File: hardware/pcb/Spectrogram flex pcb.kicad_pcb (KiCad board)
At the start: 2 copper layers, 153.2 x 54.5 mm, 10 parts

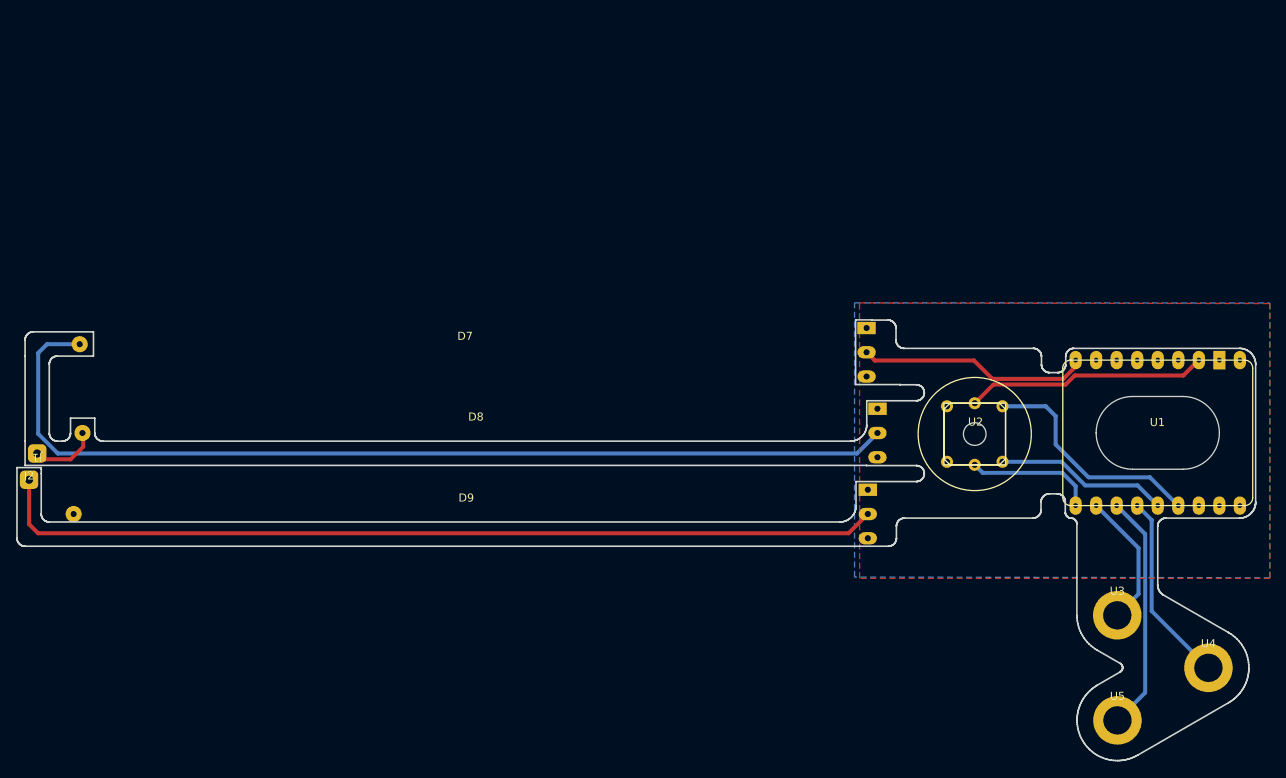
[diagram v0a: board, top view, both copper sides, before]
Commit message: PCB revision
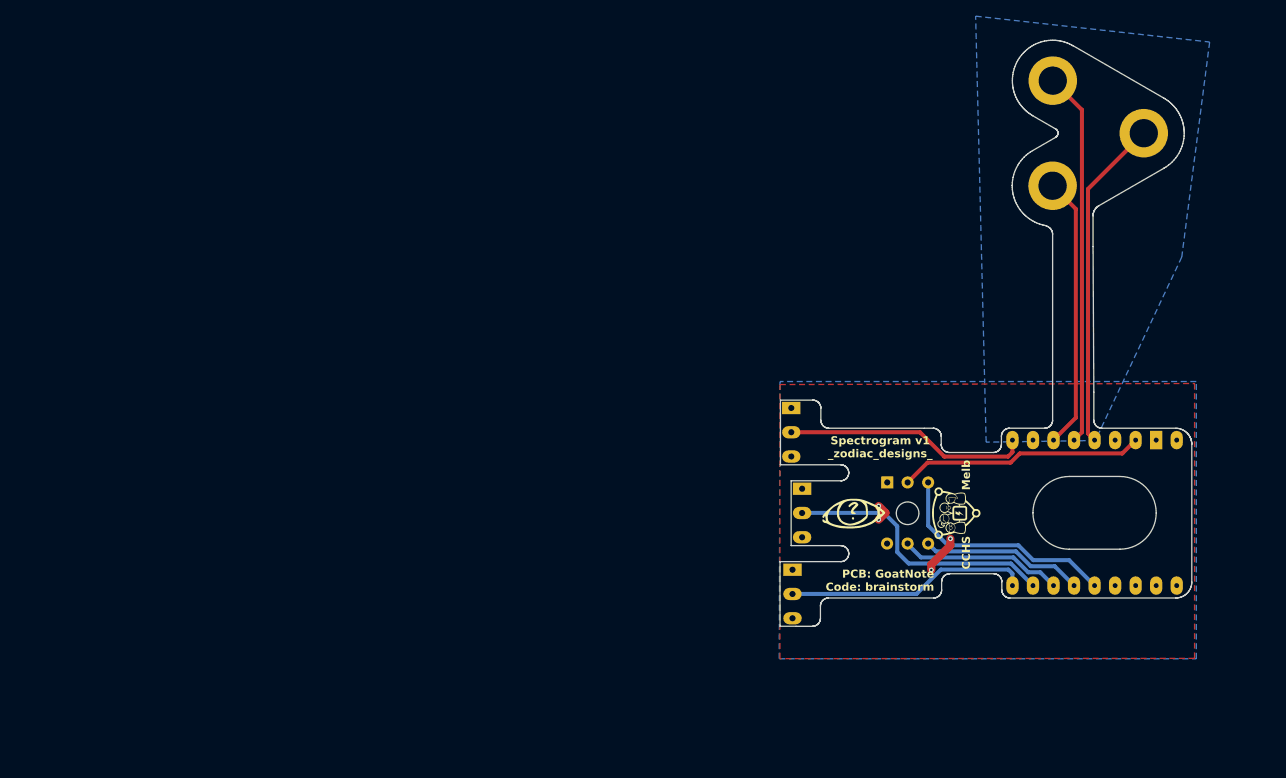
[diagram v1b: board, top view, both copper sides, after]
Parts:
- removed J1, J2: ~, Waveshare_ESP32_S3_mini:jumper pad
- added G***: LOGO, LOGO, F.Cu at (194.7, 79.2)
- added G***: LOGO, LOGO, F.Cu at (181.9, 79.4)
- added G***: LOGO, LOGO, B.Cu at (211.1, 32.4)
- moved U5 79.5 mm to (206.6, 25.7)
- moved U4 66.6 mm to (217.9, 32.2)
- moved U3 53.7 mm to (206.6, 38.7)
- moved D7 13.6 mm to (74.9, 65.2)
- moved D9 13.6 mm to (75.1, 85.2)
- moved D8 13.6 mm to (76.3, 75.2)
- moved U2 12.8 mm to (188.7, 79.2)
- moved U1 12.6 mm to (223.6, 70.1)
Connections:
- net +5V renamed Net-(D7-5V)
- D8 pad 3: Net-(D7-Dout) -> Net-(D8-Din)
- U1 pad 13: Net-(U1-GPIO12) -> unconnected-(U1-GPIO12-Pad13)
- U1 pad 17: Net-(U1-GPIO8) -> Net-(D8-Din)
- U1 pad 18: Net-(U1-GPIO7) -> Net-(D9-Din)
- U1 pad 5: unconnected-(U1-GPIO2-Pad5) -> Net-(U1-GPIO2)
- U1 pad 6: unconnected-(U1-GPIO3-Pad6) -> Net-(U1-GPIO3)
- U1 pad 7: unconnected-(U1-GPIO4-Pad7) -> Net-(U1-GPIO4)
- U2 pad 3: Net-(U1-GPIO12) -> Net-(U1-GPIO11)
- U2 pad 5: Net-(U1-GPIO7) -> Net-(U1-GPIO9)
- U2 pad 6: Net-(U1-GPIO11) -> Net-(U1-GPIO10)
- U3 pad 1: Net-(U1-GPIO8) -> Net-(U1-GPIO4)
- U4 pad 1: Net-(U1-GPIO10) -> Net-(U1-GPIO2)
- U5 pad 1: Net-(U1-GPIO9) -> Net-(U1-GPIO3)
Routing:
- net Net-(D7-Dout): track 121.5 -> 0.00 mm
- net Net-(D9-Din): track 110.7 -> 30.1 mm
- net Net-(U1-GPIO3): track 0.00 -> 46.4 mm
- net Net-(U1-GPIO2): track 0.00 -> 41.2 mm
- net Net-(D8-Din): track 0.00 -> 34.2 mm
- net Net-(U1-GPIO4): track 0.00 -> 33.8 mm
- net Net-(U1-GPIO12): track 28.9 -> 0.00 mm
- net Net-(U1-GPIO8): track 16.8 -> 0.00 mm
- net Net-(U1-GPIO7): track 16.0 -> 0.00 mm
- net Net-(U1-GPIO9): track 29.5 -> 20.2 mm
- net Net-(D8-Dout): track 9.04 -> 0.00 mm
- net Net-(U1-GPIO11): track 21.5 -> 29.0 mm
- net GND: track 0.00 -> 7.24 mm, vias 0 -> 4
- net Net-(U1-GPIO10): track 23.7 -> 20.2 mm
- net Net-(D7-Din): track 28.7 -> 30.3 mm
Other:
- board size 153.2 x 54.5 mm -> 50.9 x 72.5 mm
- board text added: "CCHS"
- board text added: "Melb"
- board text added: "PCB: GoatNote Code: brainstorm"
- board text added: "Spectrogram v1 _zodiac_designs_"
